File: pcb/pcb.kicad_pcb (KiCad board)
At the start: 2 copper layers, 77.6 x 97.5 mm, 25 parts, among them J1 Conn_02x04_Odd_Even, J10 Conn_02x04_Odd_Even, J11 Conn_02x04_Odd_Even, J12 Conn_02x04_Odd_Even, J13 Conn_02x04_Odd_Even, J14 Conn_02x04_Odd_Even, J15 Conn_02x04_Odd_Even, J16 Conn_02x04_Odd_Even, J17 Conn_02x04_Odd_Even, J18 Conn_02x04_Odd_Even, J19 Conn_02x04_Odd_Even, J2 Conn_02x04_Odd_Even, J20 Conn_02x04_Odd_Even, J21 Conn_01x05_Pin, J22 Conn_01x13_Pin, J23 Conn_01x13_Pin, J24 Conn_01x08_Pin, J25 Conn_01x16_Pin, J3 Conn_02x04_Odd_Even, J4 Conn_02x04_Odd_Even, J5 Conn_02x04_Odd_Even, J6 Conn_02x04_Odd_Even, J7 Conn_02x04_Odd_Even, J8 Conn_02x04_Odd_Even, J9 Conn_02x04_Odd_Even

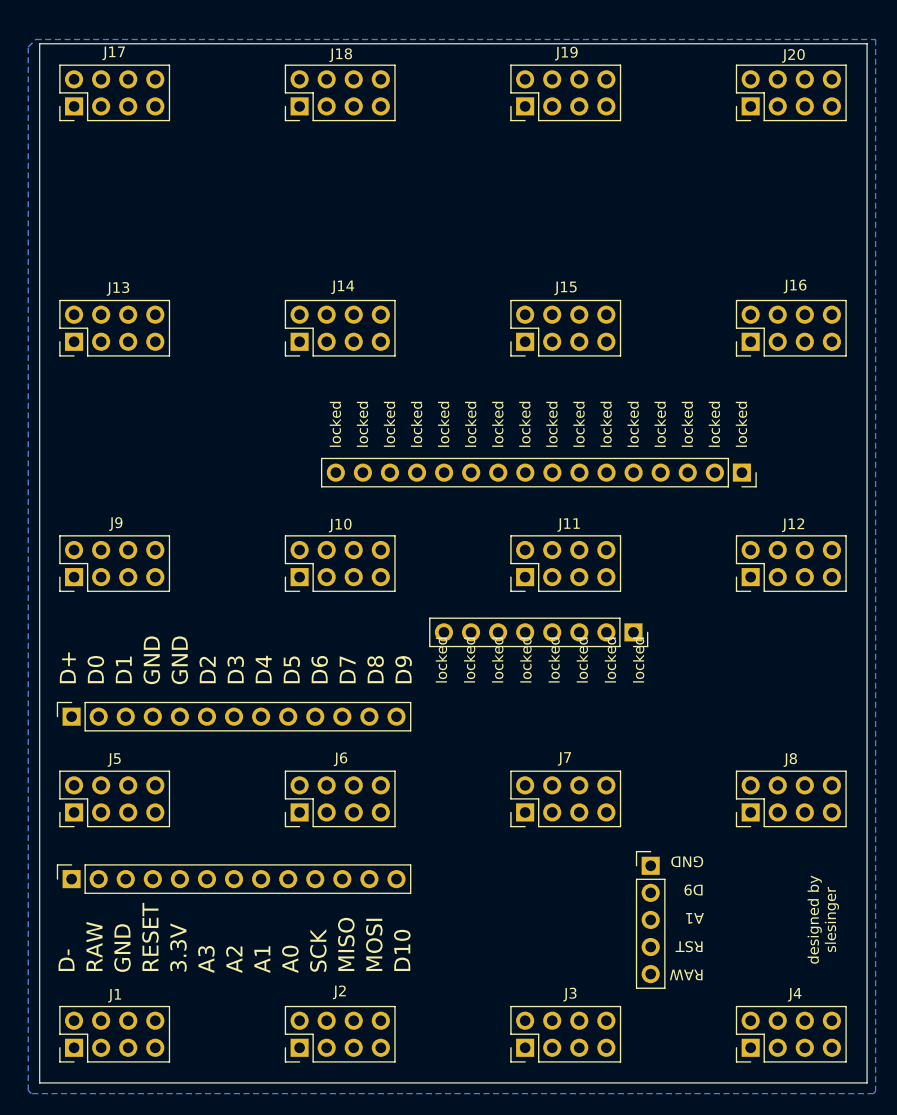
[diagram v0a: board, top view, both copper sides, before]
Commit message: updated pcb, 1x1 pcb
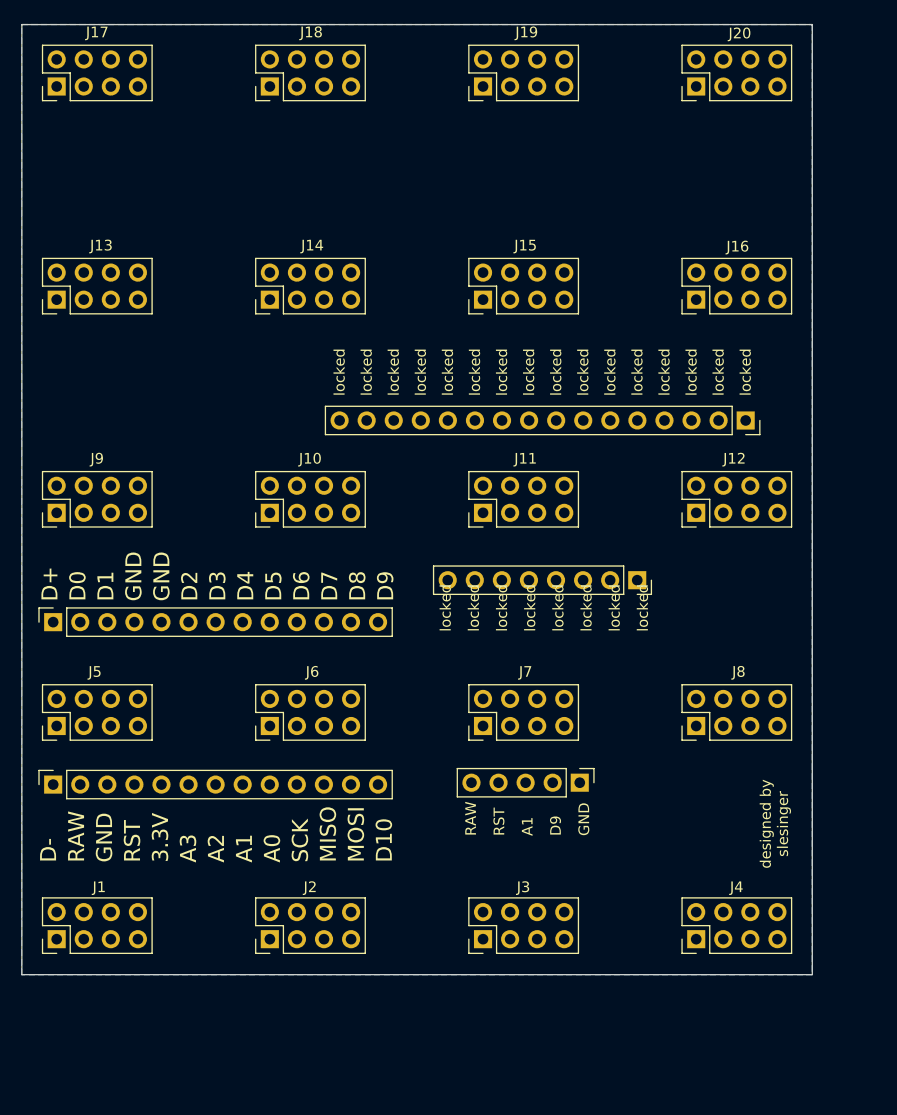
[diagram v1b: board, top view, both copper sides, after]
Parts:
- moved J4 11.4 mm to (61.3, 83.8)
- moved J3 10.9 mm to (41.3, 83.8)
- moved J2 10.6 mm to (21.3, 83.8)
- moved J1 10.3 mm to (1.27, 83.8)
- moved J21 10.2 mm to (50.3, 69.1), turned to -90 degrees
- moved J8 9.59 mm to (61.3, 63.8)
- moved J22 9.04 mm to (0.94, 54.1)
- moved J23 9.04 mm to (0.94, 69.3)
- moved J7 9.02 mm to (41.3, 63.8)
- moved J6 8.58 mm to (21.3, 63.8)
- moved J5 8.27 mm to (1.27, 63.8)
- moved J12 7.90 mm to (61.3, 43.8)
- moved J11 7.21 mm to (41.3, 43.8)
- moved J10 6.64 mm to (21.3, 43.8)
- moved J16 6.46 mm to (61.3, 23.8)
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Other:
- board size 77.6 x 97.5 mm -> 74.2 x 89.1 mm
- board text removed: "RESET"

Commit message: moved 1x1 pcb folder
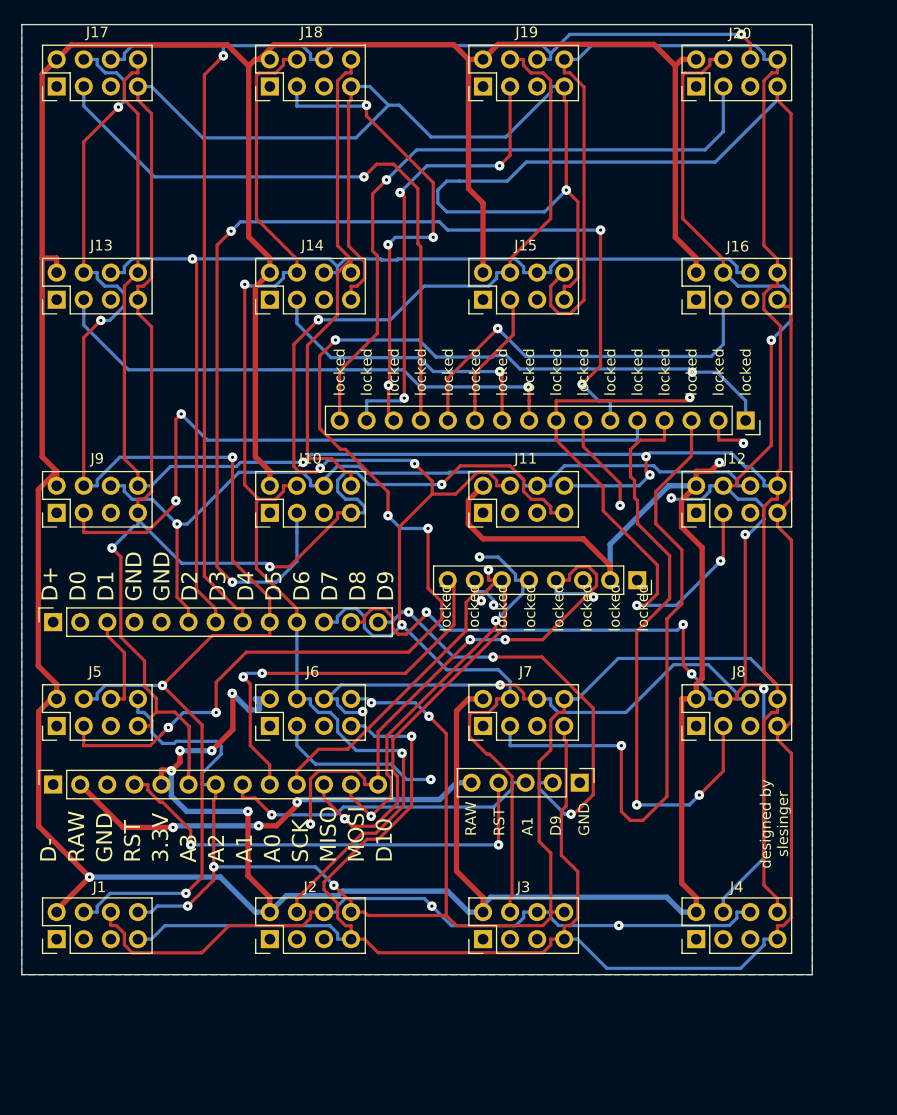
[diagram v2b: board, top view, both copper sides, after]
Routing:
- net Net-(J1-Pin_7): track 0.00 -> 481.1 mm, vias 0 -> 5
- net Net-(J1-Pin_8): track 0.00 -> 446.2 mm, vias 0 -> 8
- net +3.3V: track 0.00 -> 444.8 mm, vias 0 -> 7
- net Net-(J12-Pin_4): track 0.00 -> 153.5 mm, vias 0 -> 7
- net Net-(J11-Pin_4): track 0.00 -> 147.1 mm, vias 0 -> 4
- net Net-(J1-Pin_4): track 0.00 -> 135.7 mm, vias 0 -> 5
- net Net-(J17-Pin_6): track 0.00 -> 124.2 mm, vias 0 -> 2
- net Net-(J25-Pin_1): track 0.00 -> 118.1 mm, vias 0 -> 6
- net Net-(J10-Pin_4): track 0.00 -> 108.9 mm, vias 0 -> 2
- net Net-(J10-Pin_3): track 0.00 -> 101.2 mm, vias 0 -> 4
- net Net-(J13-Pin_6): track 0.00 -> 100.8 mm, vias 0 -> 1
- net Net-(J10-Pin_6): track 0.00 -> 79.0 mm, vias 0 -> 1
- net Net-(J1-Pin_6): track 0.00 -> 69.3 mm, vias 0 -> 2
- net Net-(J25-Pin_5): track 0.00 -> 65.9 mm, vias 0 -> 2
- net Net-(J20-Pin_3): track 0.00 -> 62.5 mm, vias 0 -> 1
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
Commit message: pcb v2
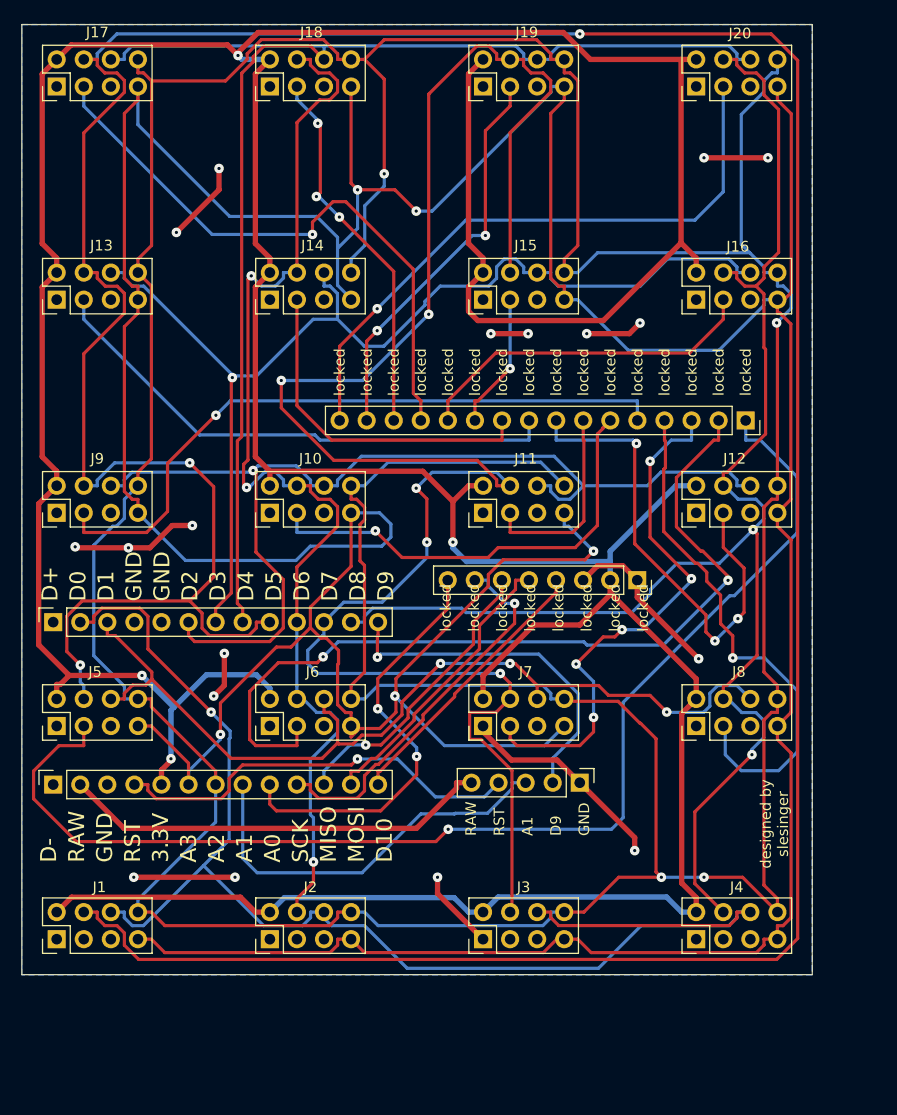
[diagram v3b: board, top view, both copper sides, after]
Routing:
- net Net-(J1-Pin_4): track 135.7 -> 328.5 mm, vias 5 -> 3
- net GND: track 0.00 -> 92.1 mm, vias 0 -> 18
- net Net-(J25-Pin_2): track 20.0 -> 79.5 mm
- net Net-(J1-Pin_6): track 69.3 -> 128.4 mm, vias 2 -> 1
- net Net-(J10-Pin_3): track 101.2 -> 42.7 mm, vias 4 -> 1
- net Net-(J11-Pin_4): track 147.1 -> 179.6 mm, vias 4 -> 5
- net Net-(J23-Pin_13): track 53.7 -> 26.3 mm, vias 4 -> 0
- net Net-(J22-Pin_3): track 59.1 -> 86.5 mm, vias 2 -> 3
- net Net-(J1-Pin_7): track 481.1 -> 453.8 mm
- net Net-(J10-Pin_6): track 79.0 -> 98.7 mm
- net Net-(J23-Pin_11): track 40.6 -> 27.8 mm, vias 3 -> 1
- net Net-(J25-Pin_3): track 62.3 -> 50.3 mm, vias 1 -> 5
- net Net-(J23-Pin_12): track 38.1 -> 27.5 mm, vias 3 -> 0
- net Net-(J12-Pin_4): track 153.5 -> 143.9 mm, vias 7 -> 2
- net Net-(J11-Pin_3): track 9.41 -> 18.7 mm, vias 1 -> 0
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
